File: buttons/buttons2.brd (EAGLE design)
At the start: 74 x 44 mm, 14 parts, among them U1 attiny2313

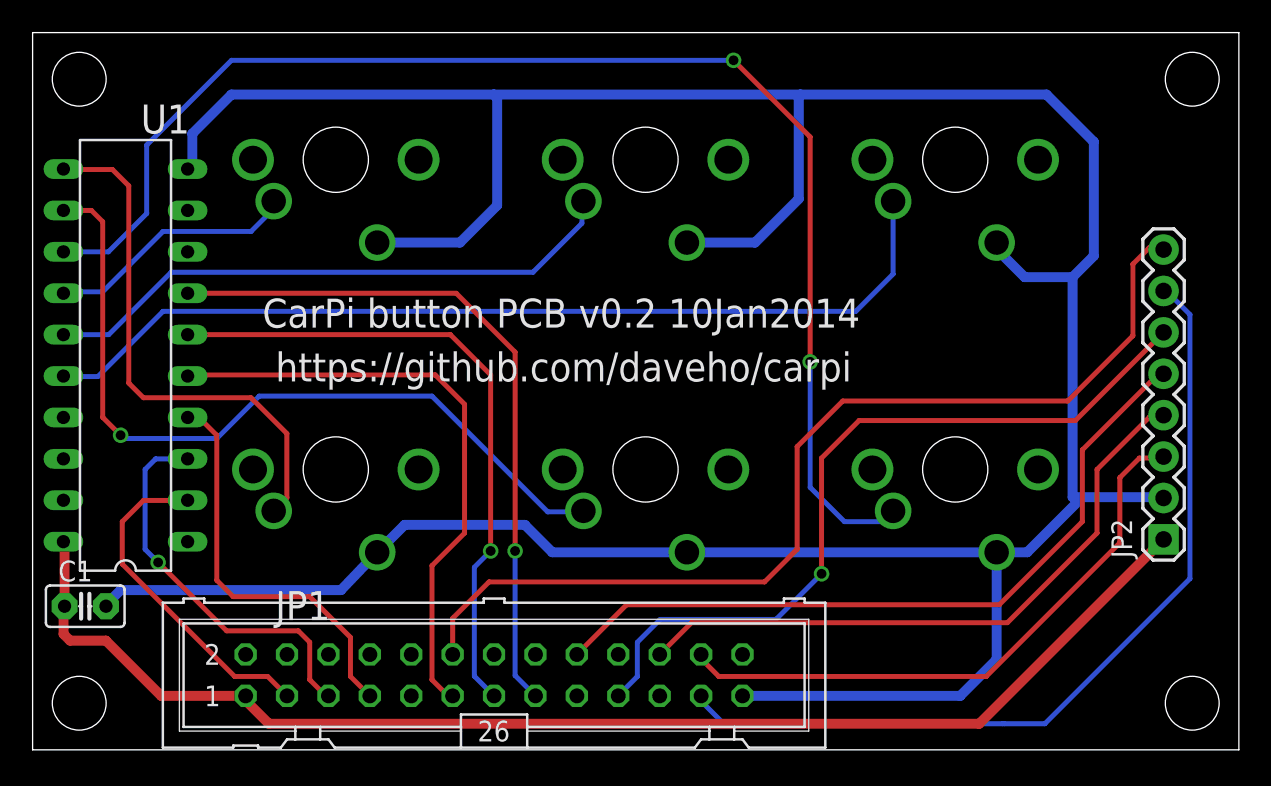
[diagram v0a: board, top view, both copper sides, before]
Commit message: a few more routing improvements
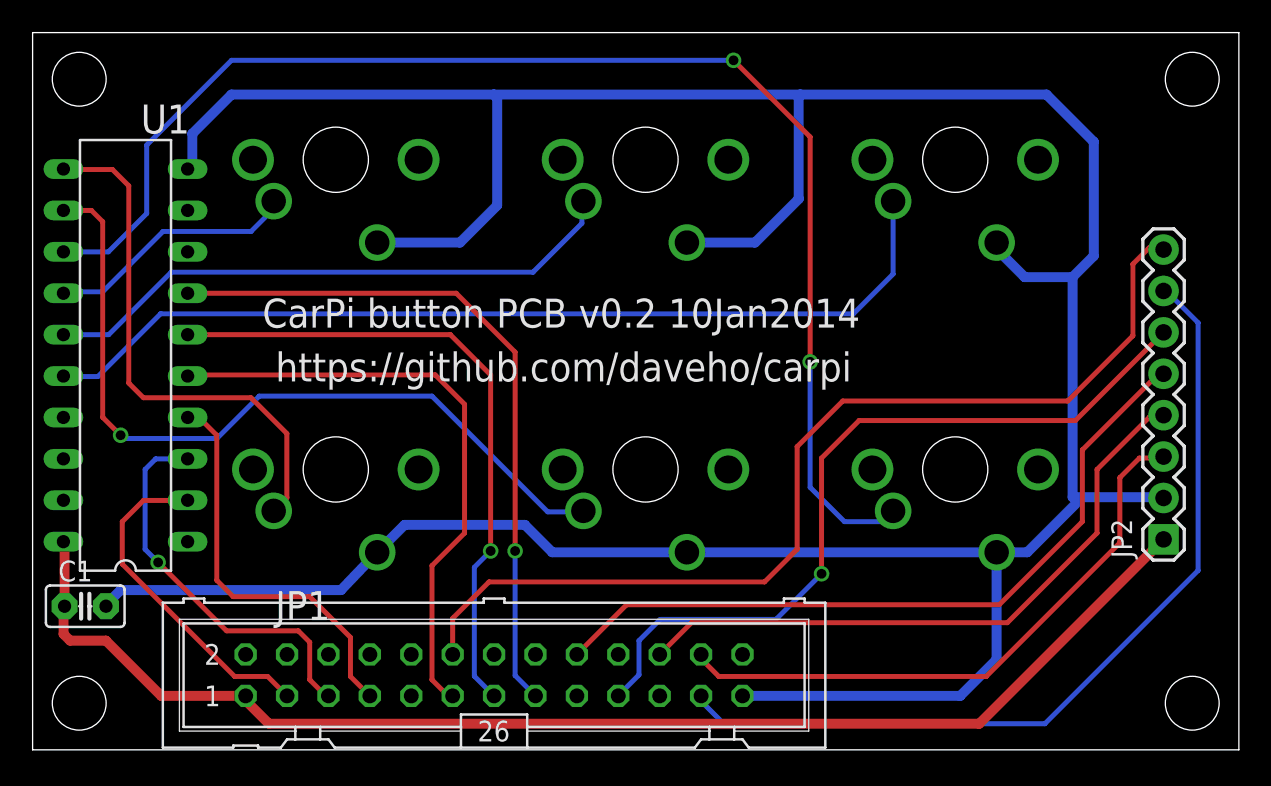
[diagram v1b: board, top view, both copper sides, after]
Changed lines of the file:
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@@
 <contactref element="S6" pad="PIN-1"/>
 <contactref element="U1" pad="16"/>
-<wire x1="52.79" y1="29.19" x2="50.5" y2="26.9" width="0.3048" layer="16"/>
-<wire x1="50.5" y1="26.9" x2="8" y2="26.9" width="0.3048" layer="16"/>
+<wire x1="52.79" y1="29.19" x2="50.35" y2="26.75" width="0.3048" layer="16"/>
 <wire x1="4" y1="22.9" x2="1.92" y2="22.9" width="0.3048" layer="16"/>
 <wire x1="1.92" y1="22.9" x2="1.89" y2="22.93" width="0.3048" layer="16"/>
-<wire x1="8" y1="26.9" x2="4" y2="22.9" width="0.3048" layer="16"/>
+<wire x1="8" y1="26.9" x2="7.85" y2="26.75" width="0" layer="19" extent="1-16"/>
+<wire x1="7.85" y1="26.75" x2="4" y2="22.9" width="0.3048" layer="16"/>
 <wire x1="52.79" y1="33.66" x2="52.79" y2="29.19" width="0.3048" layer="16"/>
+<wire x1="50.35" y1="26.75" x2="7.85" y2="26.75" width="0.3048" layer="16"/>
 </signal>
 <signal name="N$2">
@@
 <wire x1="48.4" y1="10.8" x2="45.6" y2="8" width="0.3048" layer="16"/>
 <wire x1="45.6" y1="8" x2="38.5" y2="8" width="0.3048" layer="16"/>
-<wire x1="38.5" y1="8" x2="37.1" y2="6.6" width="0.3048" layer="16"/>
-<wire x1="37.1" y1="6.6" x2="37.1" y2="4.5" width="0.3048" layer="16"/>
-<wire x1="37.1" y1="4.5" x2="35.93" y2="3.33" width="0.3048" layer="16"/>
+<wire x1="37.2" y1="4.6" x2="35.93" y2="3.33" width="0.3048" layer="16"/>
 <wire x1="35.93" y1="3.33" x2="35.93" y2="3.31" width="0.3048" layer="16"/>
+<wire x1="37.2" y1="4.6" x2="37.2" y2="6.7" width="0.3048" layer="16"/>
+<wire x1="37.2" y1="6.7" x2="38.5" y2="8" width="0.3048" layer="16"/>
 </signal>
 <signal name="SCK">
@@
 <contactref element="JP1" pad="23"/>
 <wire x1="69.38" y1="28.15" x2="69.55" y2="28.15" width="0.3048" layer="16"/>
-<wire x1="69.55" y1="28.15" x2="71" y2="26.7" width="0.3048" layer="16"/>
-<wire x1="71" y1="26.7" x2="71" y2="10.5" width="0.3048" layer="16"/>
+<wire x1="69.55" y1="28.15" x2="71.5" y2="26.2" width="0.3048" layer="16"/>
 <wire x1="41.01" y1="3.31" x2="41.01" y2="2.99" width="0.3048" layer="16"/>
 <wire x1="41.01" y1="2.99" x2="42.4" y2="1.6" width="0.3048" layer="16"/>
-<wire x1="42.4" y1="1.6" x2="59.5" y2="1.6" width="0.3048" layer="16"/>
-<wire x1="59.5" y1="1.6" x2="59.6" y2="1.6" width="0.3048" layer="16"/>
-<wire x1="71" y1="10.5" x2="62.1" y2="1.6" width="0.3048" layer="16"/>
-<wire x1="62.1" y1="1.6" x2="59.6" y2="1.6" width="0.3048" layer="16"/>
+<wire x1="42.4" y1="1.6" x2="62.1" y2="1.6" width="0.3048" layer="16"/>
+<wire x1="71.5" y1="11" x2="62.1" y2="1.6" width="0.3048" layer="16"/>
+<wire x1="71.5" y1="26.2" x2="71.5" y2="11" width="0.3048" layer="16"/>
 </signal>
 <signal name="BUTTON1">
@@
 <wire x1="27.1" y1="11.2" x2="28.1" y2="12.2" width="0.3048" layer="16"/>
 <via x="28.1" y="12.2" extent="1-16" drill="0.6"/>
-<wire x1="28.1" y1="23.8" x2="28.1" y2="23" width="0" layer="19" extent="1-16"/>
 <wire x1="28.1" y1="23" x2="28.1" y2="12.2" width="0.3048" layer="1"/>
 <wire x1="9.51" y1="25.47" x2="25.63" y2="25.47" width="0.3048" layer="1"/>
